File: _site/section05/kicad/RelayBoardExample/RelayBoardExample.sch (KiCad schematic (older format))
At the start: 9 parts

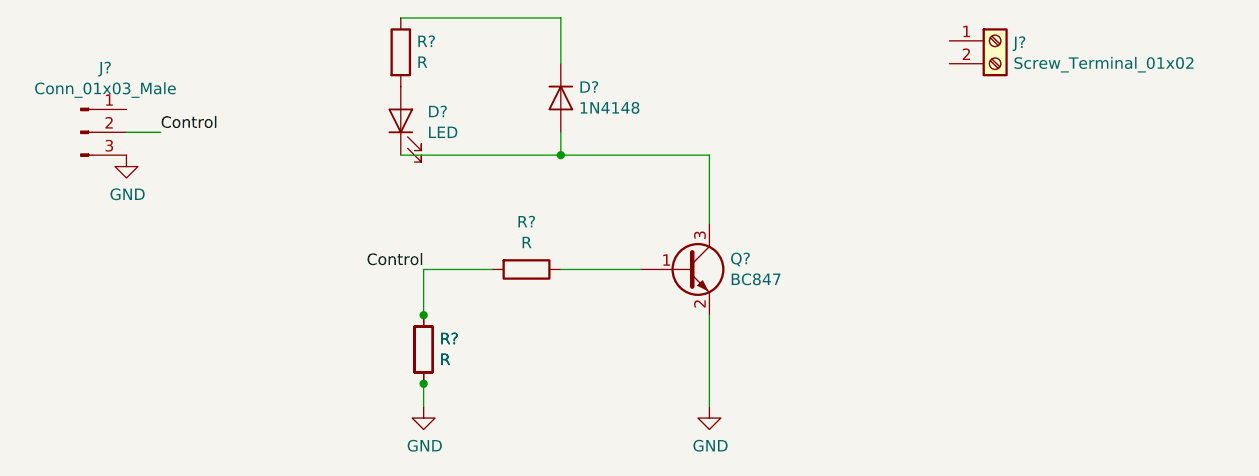
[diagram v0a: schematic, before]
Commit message: Notes for the final project.
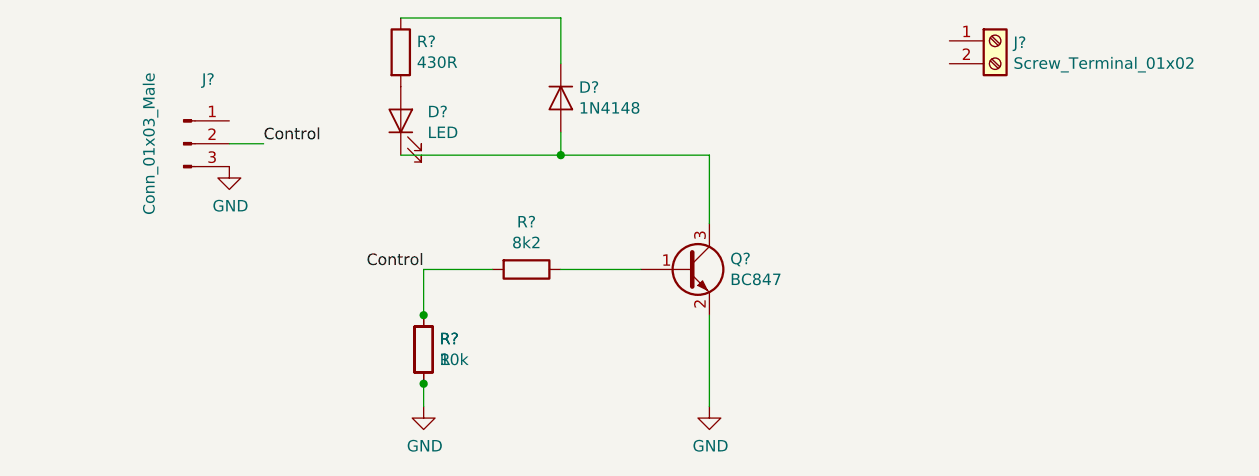
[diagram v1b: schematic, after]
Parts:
- R?: value R -> 10k
- R?: value R -> 8k2
- R?: value R -> 430R
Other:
- moved on the sheet: J?
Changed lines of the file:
@@
 P 3550 3550
 F 0 "R?" H 3620 3596 50  0000 L CNN
-F 1 "R" H 3620 3505 50  0000 L CNN
+F 1 "10k" H 3620 3505 50  0000 L CNN
 F 2 "" V 3480 3550 50  0001 C CNN
 F 3 "~" H 3550 3550 50  0001 C CNN
@@
 P 4000 3200
 F 0 "R?" V 3793 3200 50  0000 C CNN
-F 1 "R" V 3884 3200 50  0000 C CNN
+F 1 "8k2" V 3884 3200 50  0000 C CNN
 F 2 "" V 3930 3200 50  0001 C CNN
 F 3 "~" H 4000 3200 50  0001 C CNN
@@
 P 3450 2250
 F 0 "R?" H 3520 2296 50  0000 L CNN
-F 1 "R" H 3520 2205 50  0000 L CNN
+F 1 "430R" H 3520 2205 50  0000 L CNN
 F 2 "" V 3380 2250 50  0001 C CNN
 F 3 "~" H 3450 2250 50  0001 C CNN
@@
 L Connector:Conn_01x03_Male J?
 U 1 1 5E852703
-P 2050 2600
-F 0 "J?" H 2158 2881 50  0000 C CNN
-F 1 "Conn_01x03_Male" H 2158 2790 50  0000 C CNN
-F 2 "" H 2050 2600 50  0001 C CNN
-F 3 "~" H 2050 2600 50  0001 C CNN
-	1    2050 2600
+P 2500 2650
+F 0 "J?" H 2608 2931 50  0000 C CNN
+F 1 "Conn_01x03_Male" V 2350 2650 50  0000 C CNN
+F 2 "" H 2500 2650 50  0001 C CNN
+F 3 "~" H 2500 2650 50  0001 C CNN
+	1    2500 2650
 	1    0    0    -1
 $EndComp
@@
 Connection ~ 4150 2700
 $Comp
-L power:GND #PWR?
+L power:GND #PWR0101
 U 1 1 5E85F1FA
 P 3550 3800
-F 0 "#PWR?" H 3550 3550 50  0001 C CNN
+F 0 "#PWR0101" H 3550 3550 50  0001 C CNN
 F 1 "GND" H 3555 3627 50  0000 C CNN
 F 2 "" H 3550 3800 50  0001 C CNN
@@
 $EndComp
 $Comp
-L power:GND #PWR?
+L power:GND #PWR0102
 U 1 1 5E85F90F
-P 2250 2700
-F 0 "#PWR?" H 2250 2450 50  0001 C CNN
-F 1 "GND" H 2255 2527 50  0000 C CNN
-F 2 "" H 2250 2700 50  0001 C CNN
-F 3 "" H 2250 2700 50  0001 C CNN
-	1    2250 2700
+P 2700 2750
+F 0 "#PWR0102" H 2700 2500 50  0001 C CNN
+F 1 "GND" H 2705 2577 50  0000 C CNN
+F 2 "" H 2700 2750 50  0001 C CNN
+F 3 "" H 2700 2750 50  0001 C CNN
+	1    2700 2750
 	1    0    0    -1
 $EndComp
 $Comp
-L power:GND #PWR?
+L power:GND #PWR0103
 U 1 1 5E860052
 P 4800 3800
-F 0 "#PWR?" H 4800 3550 50  0001 C CNN
+F 0 "#PWR0103" H 4800 3550 50  0001 C CNN
 F 1 "GND" H 4805 3627 50  0000 C CNN
 F 2 "" H 4800 3800 50  0001 C CNN
@@
 Wire Wire Line
 	4800 3800 4800 3400
-Text Label 2400 2600 0    50   ~ 0
+Text Label 2850 2650 0    50   ~ 0
 Control
 Wire Wire Line
-	2250 2600 2400 2600
+	2700 2650 2850 2650
 Text Label 3550 3200 2    50   ~ 0
 Control
